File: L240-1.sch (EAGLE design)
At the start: 15 parts, among them IC1 TINY13-20SSU, IC2 LM1117IMPX-3.3, K1 G6RW, X1 MKDSN1,5/2-5,08, X2 22-23-2021, X3 MKDSN1,5/2-5,08

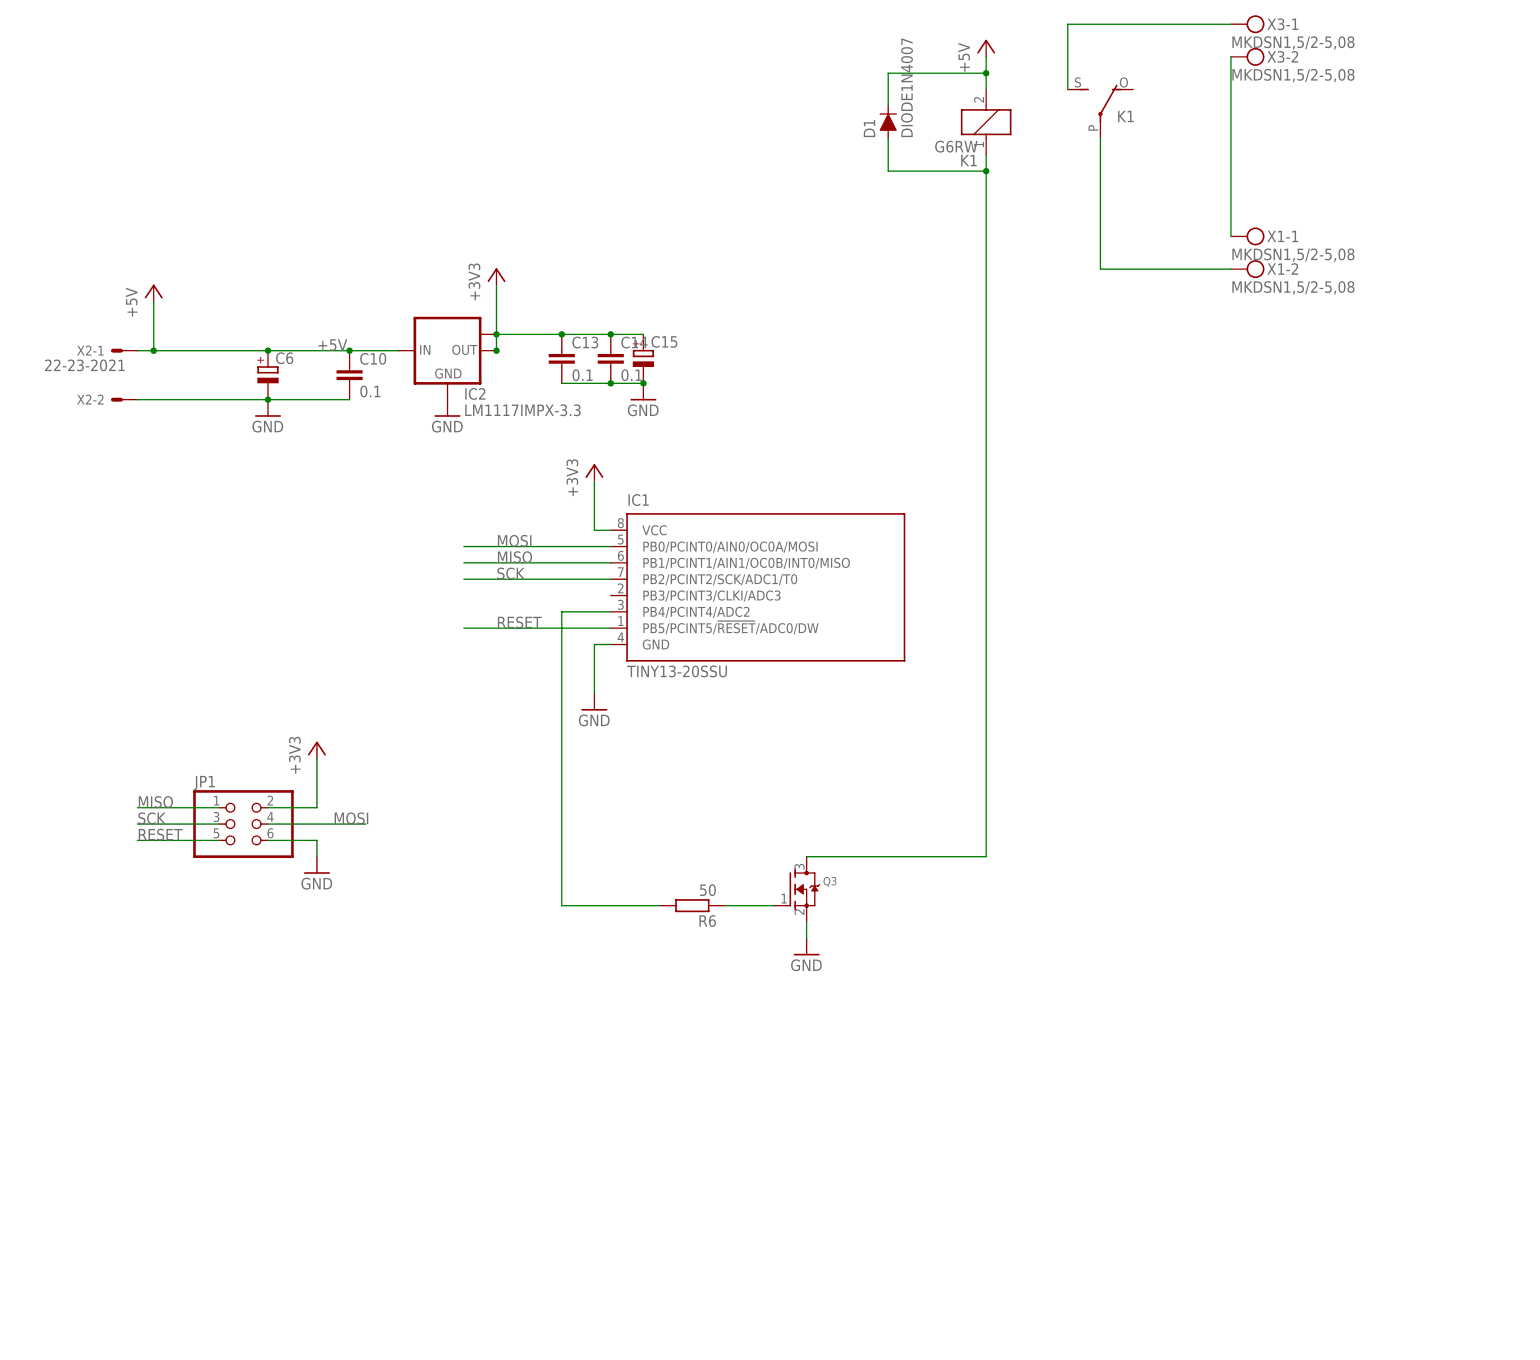
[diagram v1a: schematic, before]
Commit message: wip
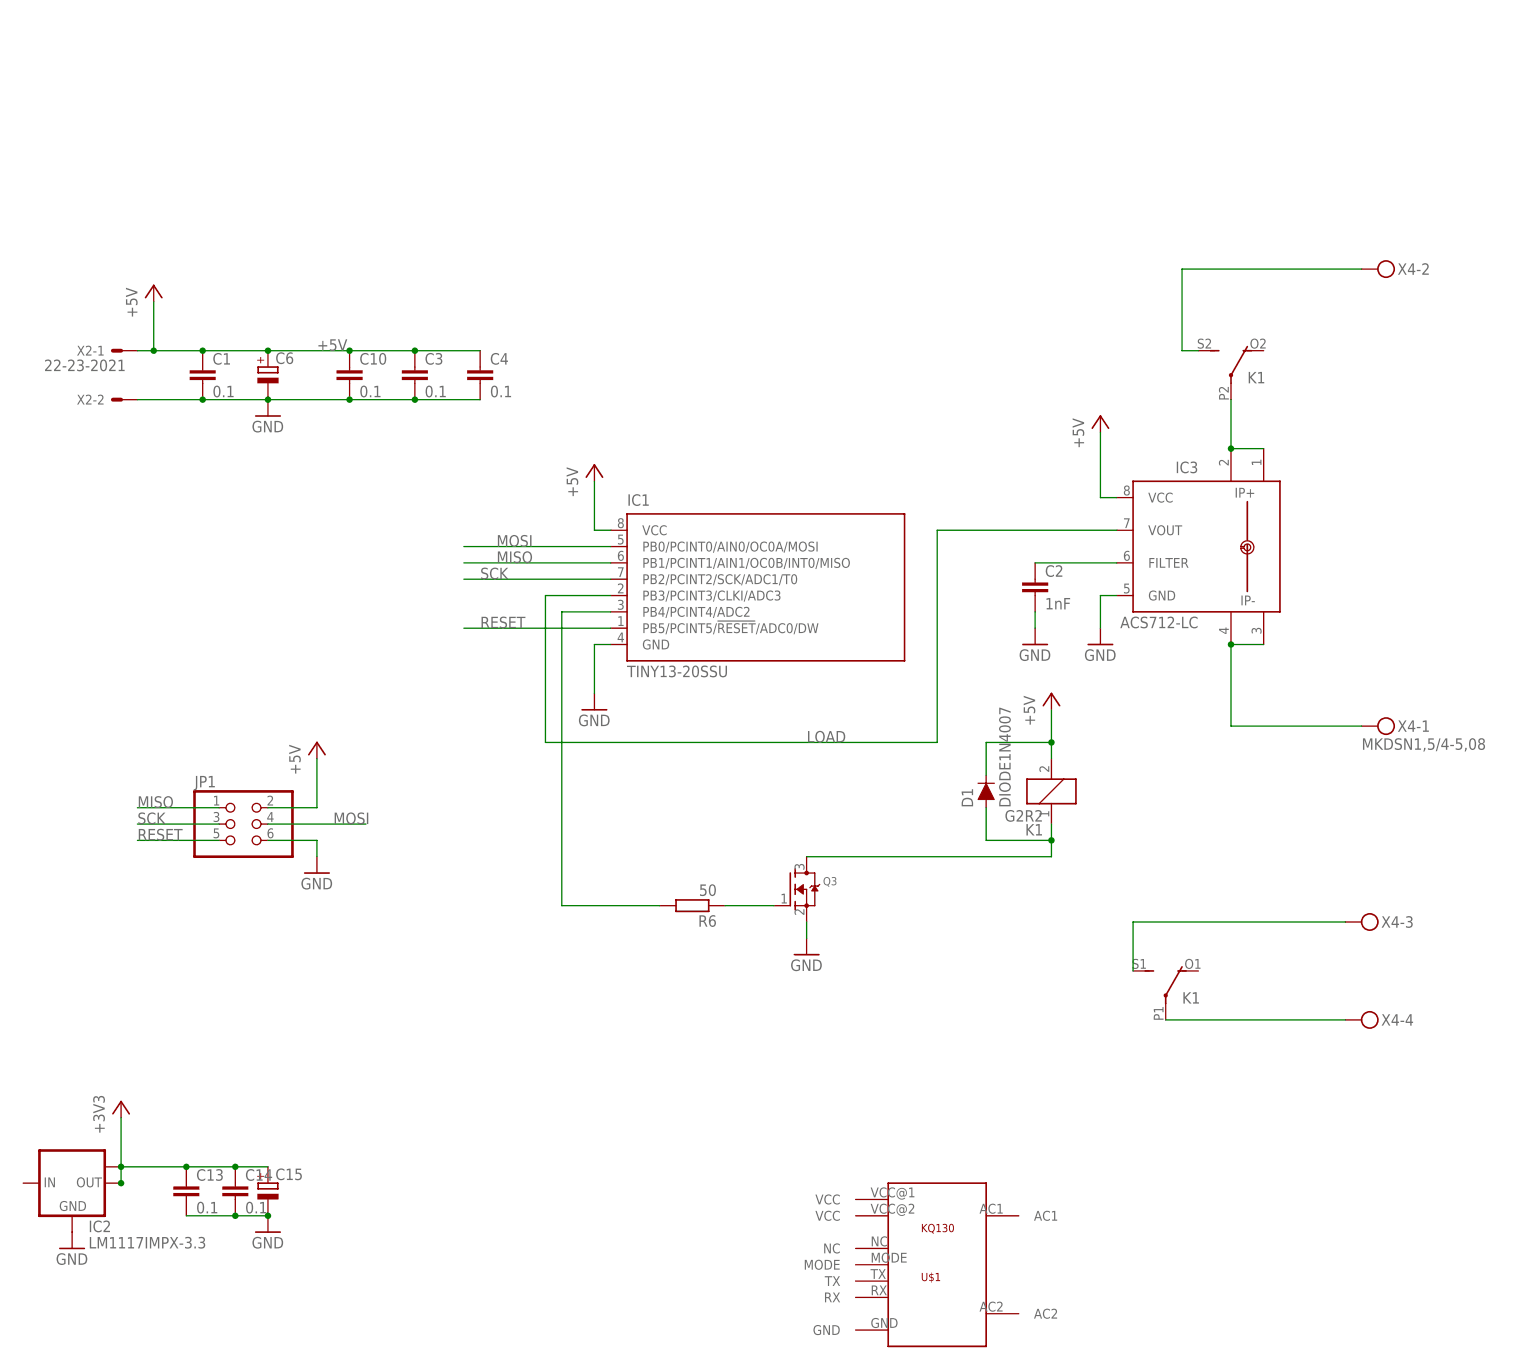
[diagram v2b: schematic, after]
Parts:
- removed X1, X3: MKDSN1,5/2-5,08, con-phoenix-508:MKDSN1,5/2-5,08
- added C1, C3, C4: 0.1, rcl:C-EUC0805
- added C2: 1nF, rcl:C-EUC0805
- added IC3: ACS712-LC, allegro-2:ACS712-LC
- added U$1: KQ130, MyLib:KQ130
- added X4: MKDSN1,5/4-5,08, con-phoenix-508:MKDSN1,5/4-5,08
- K1: value G6RW -> G2R2; device relay:G6RW -> relay:G2R2
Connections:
- new net LOAD: IC1.PB3/PCINT3/CLKI/ADC3, IC3.VOUT
- new net N$4: IC3.IP-, IC3.IP-1, X4-1.KL
- new net N$6: K13.S, X4-2.KL
- new net N$7: C2.1, IC3.FILTER
- net +3V3: no longer IC1.VCC, JP1.2
- net +5V: now also C1.1, C3.1, C4.1, IC1.VCC, IC3.VCC, JP1.2; no longer IC2.IN
- net GND: now also C1.2, C2.2, C3.2, C4.2, IC3.GND
- net N$1: now also K12.S, X4-3.KL; no longer X1-1.KL, X3-2.KL
- net N$2: now also IC3.IP+, IC3.IP+1, K13.P; no longer K12.S, X3-1.KL
- net N$3: now also X4-4.KL; no longer X1-2.KL
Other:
- moved on the sheet: C13, C14, C15, D1, IC2, K1
